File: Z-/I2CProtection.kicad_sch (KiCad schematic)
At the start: 9 parts, among them Q3 NX3008NBKS, Q4 MBT2222ADW1T1

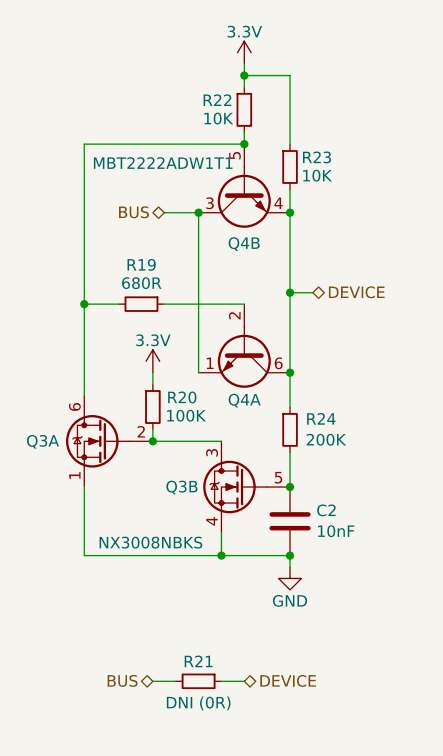
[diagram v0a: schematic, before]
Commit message: temp
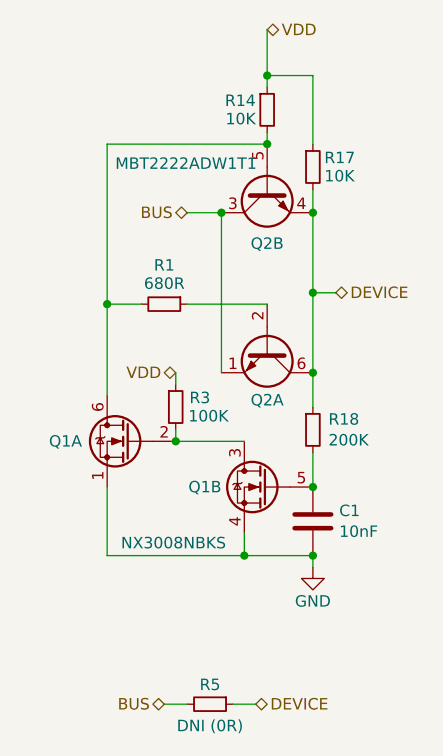
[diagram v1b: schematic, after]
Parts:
- removed C2: 10nF, Capacitor_SMD:C_0603_1608Metric, symbol Device:C
- removed Q3: NX3008NBKS, Package_TO_SOT_SMD:SOT-363_SC-70-6, symbol Argus-Miscellaneous:NX3008NBKS
- removed Q4: MBT2222ADW1T1, Package_TO_SOT_SMD:SOT-363_SC-70-6, symbol Transistor_BJT:MBT2222ADW1T1
- removed R19: 680R, Resistor_SMD:R_0603_1608Metric, symbol Device:R_Small
- removed R20: 100K, Resistor_SMD:R_0603_1608Metric, symbol Device:R_Small
- removed R21: DNI (0R), Resistor_SMD:R_0603_1608Metric, symbol Device:R_Small
- removed R22, R23: 10K, Resistor_SMD:R_0603_1608Metric, symbol Device:R_Small
- removed R24: 200K, Resistor_SMD:R_0603_1608Metric, symbol Device:R_Small
- added C1: 10nF, Capacitor_SMD:C_0603_1608Metric, symbol Device:C
- added Q1: NX3008NBKS, Package_TO_SOT_SMD:SOT-363_SC-70-6, symbol Argus-Miscellaneous:NX3008NBKS
- added Q2: MBT2222ADW1T1, Package_TO_SOT_SMD:SOT-363_SC-70-6, symbol Transistor_BJT:MBT2222ADW1T1
- added R1: 680R, Resistor_SMD:R_0603_1608Metric, symbol Device:R_Small
- added R14, R17: 10K, Resistor_SMD:R_0603_1608Metric, symbol Device:R_Small
- added R18: 200K, Resistor_SMD:R_0603_1608Metric, symbol Device:R_Small
- added R3: 100K, Resistor_SMD:R_0603_1608Metric, symbol Device:R_Small
- added R5: DNI (0R), Resistor_SMD:R_0603_1608Metric, symbol Device:R_Small
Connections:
- net BUS: now also Q2.1 (E1), Q2.3 (C2), R5.2
- net DEVICE: now also Q2.4 (E2), Q2.6 (C1), R17.2, R18.1, R5.1
- net GND: now also C1.2, Q1.1 (S2), Q1.4 (S1)
- new net: Q1.6 (D1), Q2.5 (B2), R1.2, R14.2
- new net: Q2.2 (B1), R1.1
- new net: C1.1, Q1.5 (G1), R18.2
- new net: Q1.2 (G2), Q1.3 (D2), R3.2
- new net VDD: R14.1, R17.1, R3.1
